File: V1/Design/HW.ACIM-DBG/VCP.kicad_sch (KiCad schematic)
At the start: 51 parts, among them Q1 MFET N, U10 12MHz, U3 SPI EEPROM, U8 FT4232H, U9 SHIFT REG 8BIT

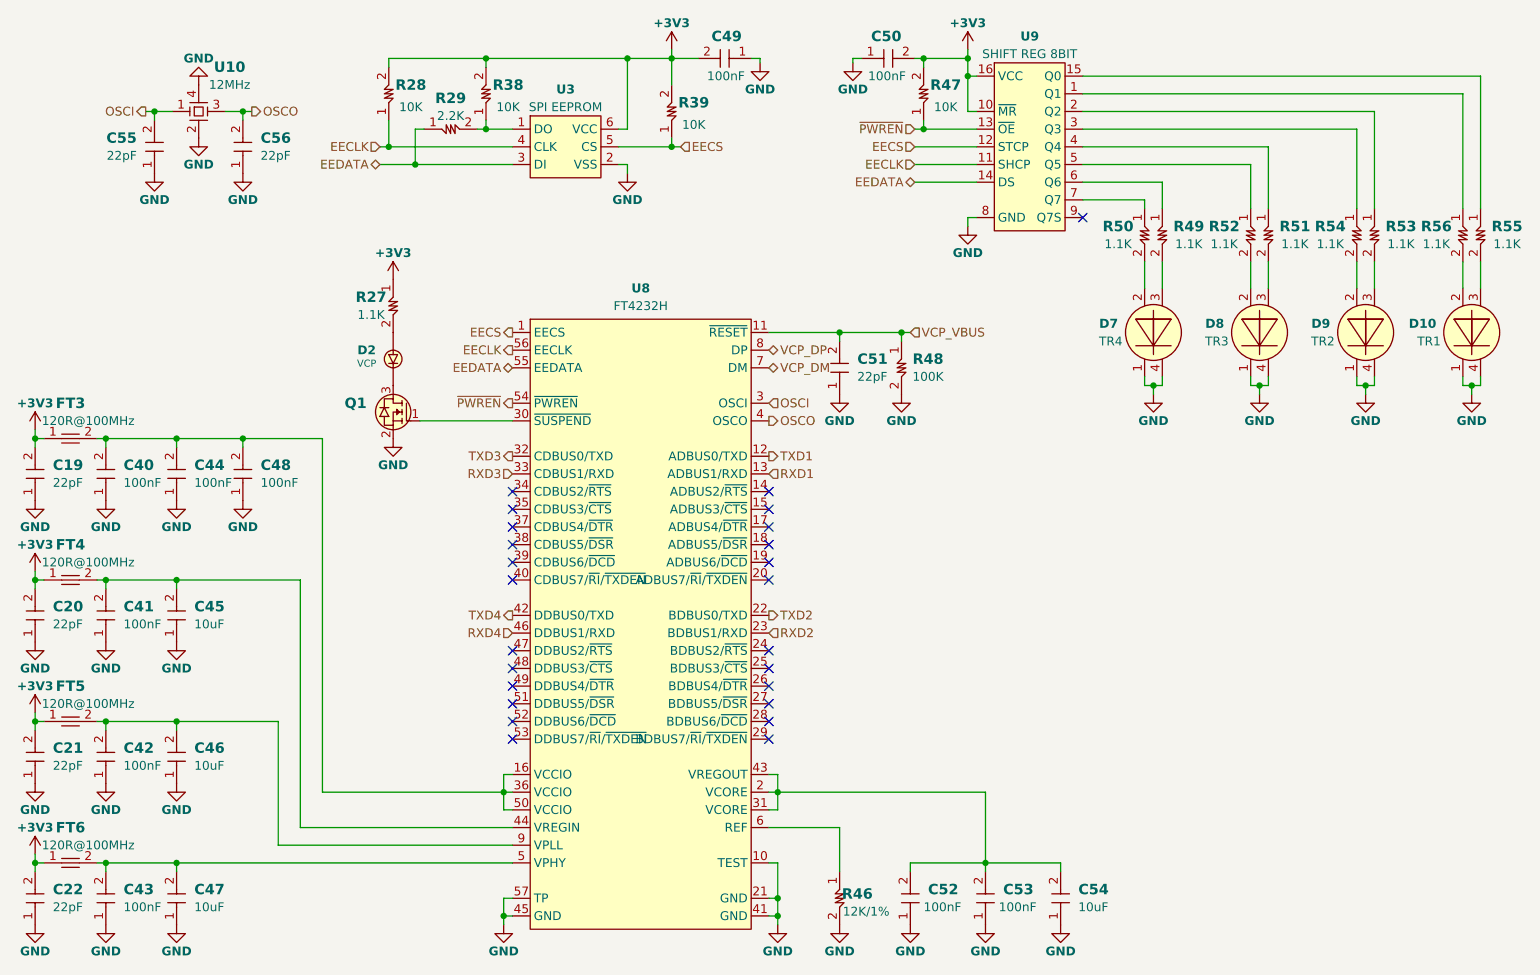
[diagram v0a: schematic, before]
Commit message: V1 layout update 8
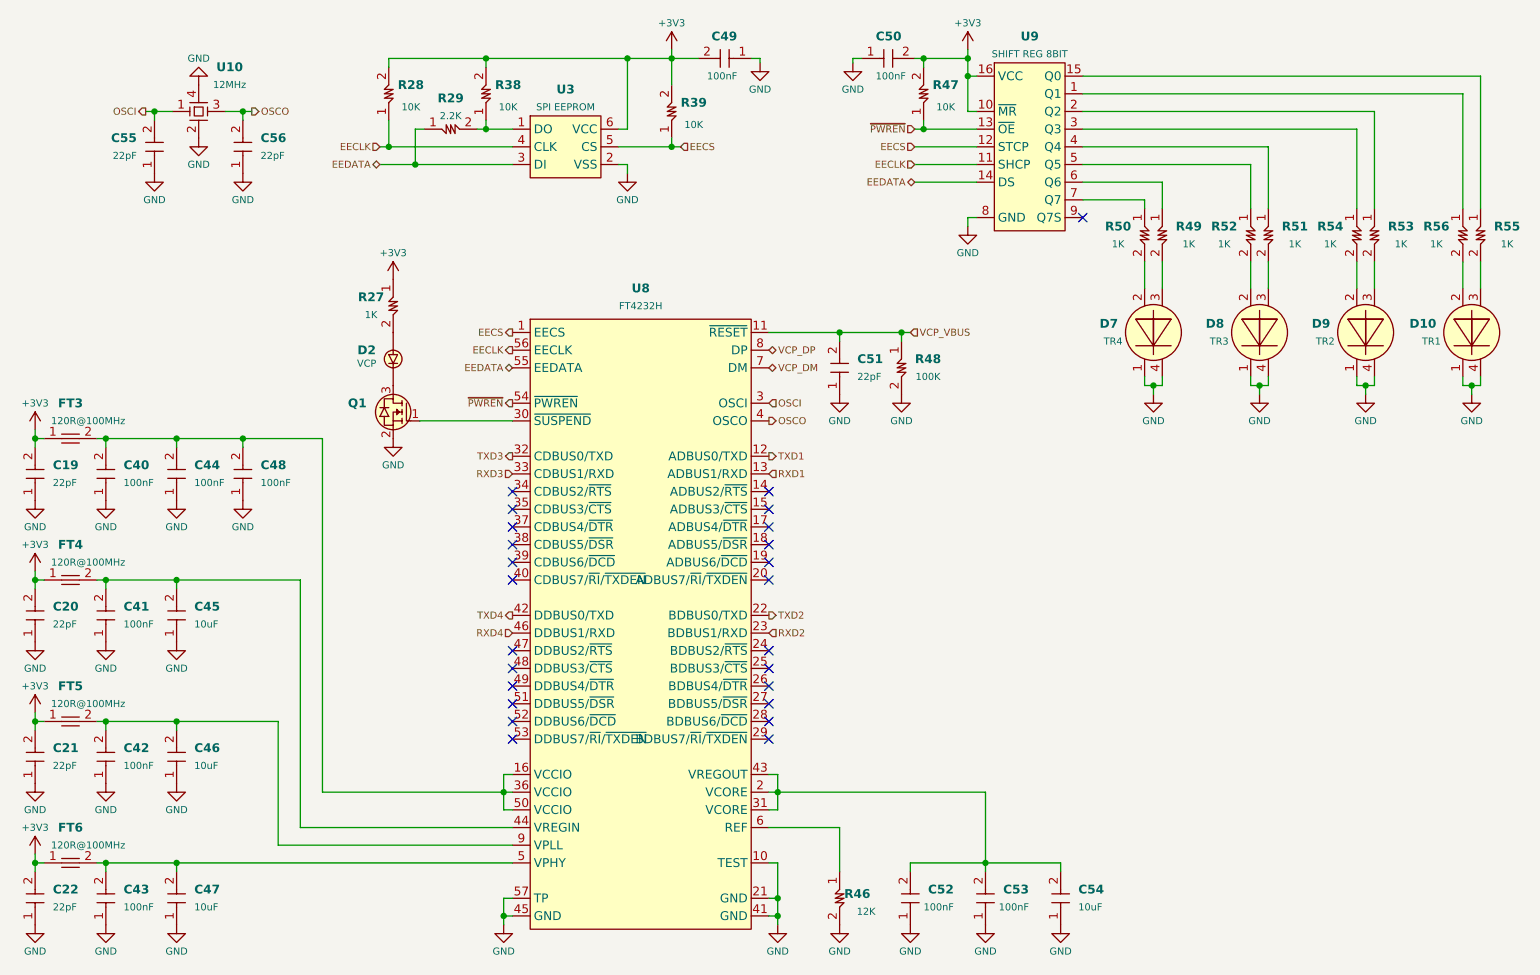
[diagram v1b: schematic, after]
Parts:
- C19, C20, C21, C22, C51, C55, C56: MFT Walsin -> YAGE; MNP 0603N220J500CT -> CC0603JRNPO9BN220
- C40, C41, C42, C43, C44, C48, C49, C50, C52, C53: MFT Samsung -> YAGE; MNP CL10B104KB8NNNC -> CC0603ZRY5V9BB104
- C45, C46, C47, C54: MFT Samsung -> TAIY; MNP CL10A106MQ8NNNC -> EMK107BBJ106MA-T
- D10, D7, D8, D9: MFT Harvatek -> ROHM; MNP B2612USNG20D000212U1930 -> SML-522MU8WT86
- D2: MFT Würth Elektronik -> ROHM; MNP 151031VS06000 -> SML-D12M8WT86
- FT3, FT4, FT5, FT6: MFT Pulse -> TDK; MNP PE-0603PFB121ST -> MPZ1608S121ATAH0
- Q1: MFT VISHAY -> IRF; MNP SI2318CDS-T1-GE3 -> IRLML2402GTRPBF
- R27, R49, R50, R51, R52, R53, R54, R55, R56: value 1.1K -> 1K; MFT YAGEO -> ROHM; MNP AC0603FR-071K1L -> MCR03PZPZFX1001
- R46: value 12K/1% -> 12K
- R48: MFT YAGEO -> NIC; MNP RC0603FR-07100KL -> NRC06F1003TRF
- U10: MFT Abracon LLC -> ABRC; MNP ABM10AIG-12.000MHZ-4Z-T3 -> ABM10-167-12.000MHZ-T3
- U9: MFT Nexperia -> FCS; MNP 74HC595PW,118 -> MM74HC595MX
